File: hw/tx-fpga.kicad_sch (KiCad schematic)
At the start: 12 parts, among them U2401 ICE40UP3K-UWG30ITR1K

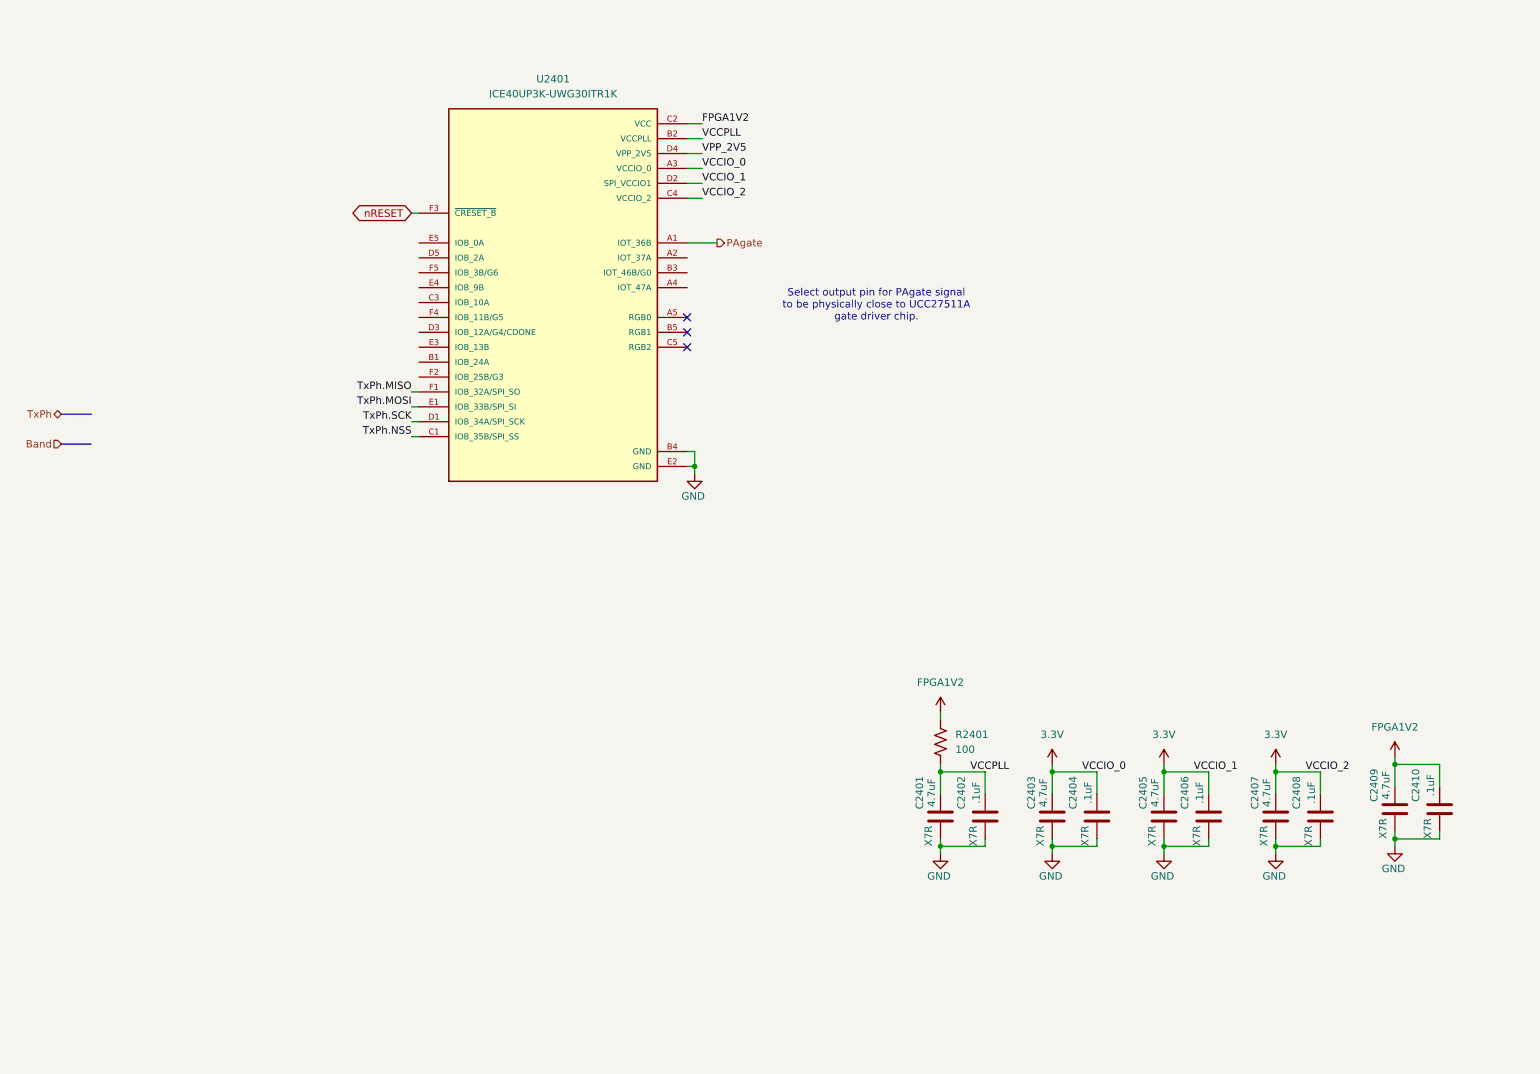
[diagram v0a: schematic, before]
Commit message: Checkpoint
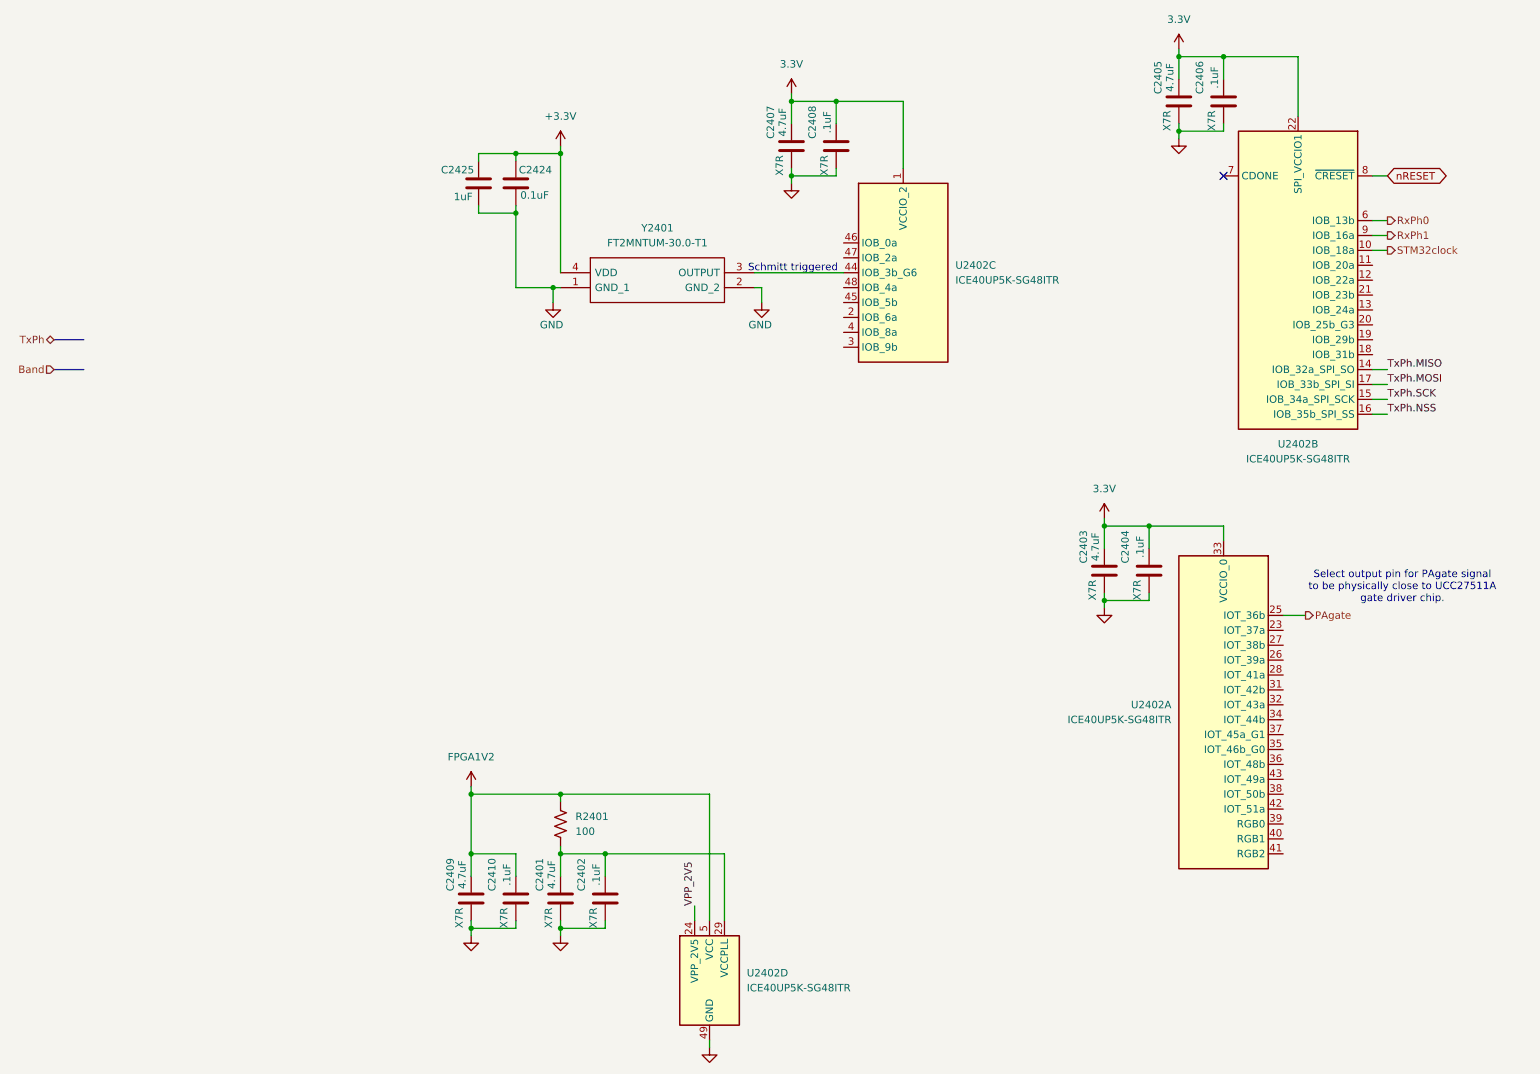
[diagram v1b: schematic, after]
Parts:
- removed U2401: ICE40UP3K-UWG30ITR1K, ICE40UP3K-UWG30ITR1K:BGA30N40P6X5_253X211X60N, symbol ICE40UP3K-UWG30ITR1K:ICE40UP3K-UWG30ITR1K
- added C2424: 0.1uF, symbol Device:C
- added C2425: 1uF, symbol Device:C
- added U2402: ICE40UP5K-SG48ITR, Package_DFN_QFN:QFN-48-1EP_7x7mm_P0.5mm_EP5.6x5.6mm, symbol FPGA_Lattice:ICE40UP5K-SG48ITR
- added Y2401: FT2MNTUM-30.0-T1, FT2MNTUM300T1, symbol FT2MNTUM-30.0-T1:FT2MNTUM-30.0-T1
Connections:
- net 3.3V: now also U2402.1 (VCCIO_2), U2402.22 (SPI_VCCIO1), U2402.33 (VCCIO_0)
- net FPGA1V2: now also U2402.30 (VCC), U2402.5 (VCC)
- net GND: now also C2424.2, C2425.2, U2402.49 (GND), Y2401.1 (GND_1), Y2401.2 (GND_2)
- net PAgate: now also U2402.25 (IOT_36b)
- net TxPh.MISO: now also U2402.14 (IOB_32a_SPI_SO)
- net TxPh.MOSI: now also U2402.17 (IOB_33b_SPI_SI)
- net TxPh.NSS: now also U2402.16 (IOB_35b_SPI_SS)
- net TxPh.SCK: now also U2402.15 (IOB_34a_SPI_SCK)
- net VPP_2V5: now also U2402.24 (VPP_2V5)
- net nRESET: now also U2402.8 (~{CRESET})
- net VCCPLL: no longer names the net of C2401.1, C2402.1, R2401.2
- net VCCPLL: now also U2402.29 (VCCPLL)
- new net: U2402.44 (IOB_3b_G6), Y2401.3 (OUTPUT)
- new net +3.3V: C2424.1, C2425.1, Y2401.4 (VDD)
- new net RxPh0: U2402.6 (IOB_13b)
- new net RxPh1: U2402.9 (IOB_16a)
- new net STM32clock: U2402.10 (IOB_18a)
- no-connect marks 3 -> 1
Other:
- note added: "Schmitt triggered"
- moved on the sheet: C2401, C2402, C2403, C2404, C2405, C2406, C2407, C2408, C2409, C2410, R2401
